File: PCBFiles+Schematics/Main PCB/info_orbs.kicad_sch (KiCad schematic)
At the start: 11 parts, among them SW1 SW_Push, SW2 SW_Push, SW3 SW_Push

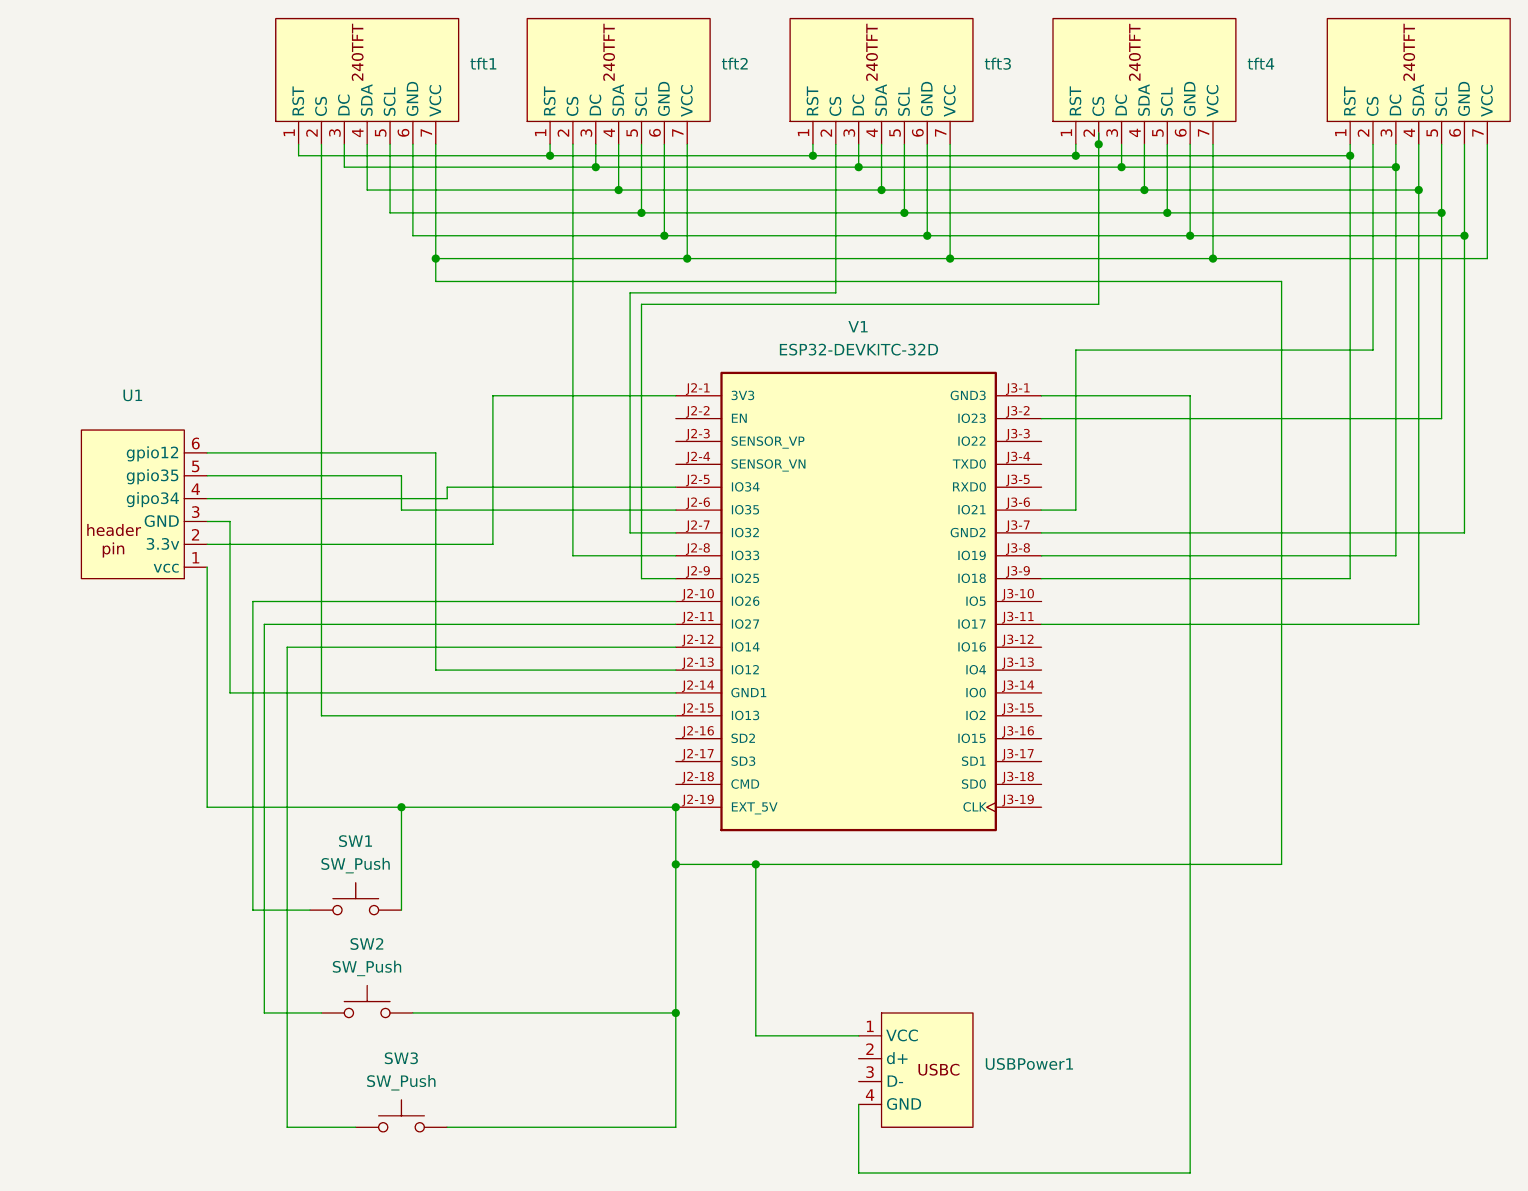
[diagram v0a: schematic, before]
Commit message: Updated New PCB Files
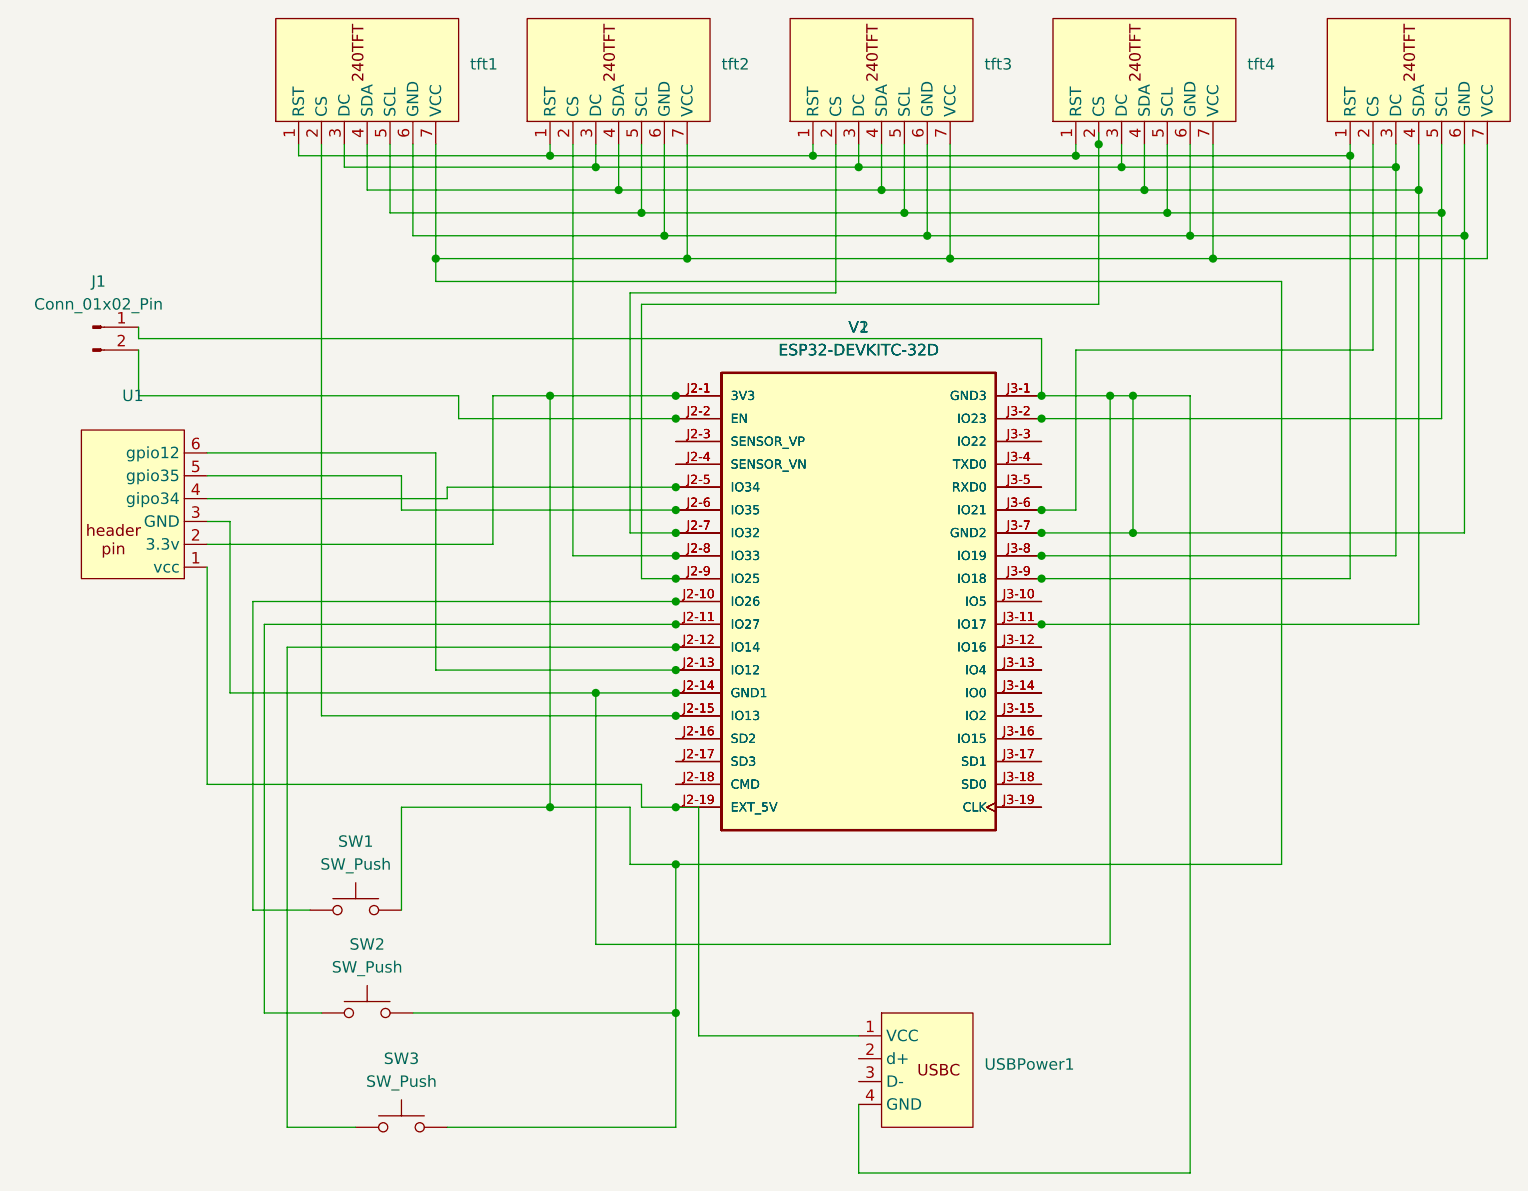
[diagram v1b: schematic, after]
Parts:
- added J1: Conn_01x02_Pin, Connector_PinHeader_2.54mm:PinHeader_1x02_P2.54mm_Vertical, symbol Connector:Conn_01x02_Pin
- added V2: ESP32-DEVKITC-32D, A Local Libs:38 Pin Board thin, symbol ESP32-DEVKITC-32D:ESP32-DEVKITC-32D
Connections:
- net at V1.J3-9 (IO18), tft1.1 (RST), tft2.1 (RST)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: now also V2.J3-9 (IO18)
- net at V1.J3-6 (IO21), tft5.2 (CS): now also V2.J3-6 (IO21)
- net at V1.J3-8 (IO19), tft1.3 (DC), tft2.3 (DC)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: now also V2.J3-8 (IO19)
- net at V1.J3-11 (IO17), tft1.4 (SDA), tft2.4 (SDA)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: now also V2.J3-11 (IO17)
- net at V1.J3-2 (IO23), tft1.5 (SCL), tft2.5 (SCL)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: now also V2.J3-2 (IO23)
- net at V1.J3-7 (GND2), tft1.6 (GND), tft2.6 (GND)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: now also U1.3 (GND), USBPower1.4 (GND), V1.J2-14 (GND1), V1.J3-1 (GND3), J1.1 (Pin_1), V2.J2-14 (GND1), V2.J3-1 (GND3), V2.J3-7 (GND2)
- net at SW1.2, SW2.2, SW3.2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: now also U1.2 (3.3v), V1.J2-1 (3V3), V2.J2-1 (3V3); no longer U1.1 (vcc), USBPower1.1 (VCC), V1.J2-19 (EXT_5V)
- net at V1.J2-7 (IO32), tft3.2 (CS): now also V2.J2-7 (IO32)
- net at U1.4 (gipo34), V1.J2-5 (IO34): now also V2.J2-5 (IO34)
- net at U1.5 (gpio35), V1.J2-6 (IO35): now also V2.J2-6 (IO35)
- net at U1.6 (gpio12), V1.J2-13 (IO12): now also V2.J2-13 (IO12)
- net at V1.J2-9 (IO25), tft4.2 (CS): now also V2.J2-9 (IO25)
- net at SW1.1, V1.J2-10 (IO26): now also V2.J2-10 (IO26)
- net at SW2.1, V1.J2-11 (IO27): now also V2.J2-11 (IO27)
- net at SW3.1, V1.J2-12 (IO14): now also V2.J2-12 (IO14)
- net at V1.J2-15 (IO13), tft1.2 (CS): now also V2.J2-15 (IO13)
- net at V1.J2-16 (SD2): now also V2.J2-16 (SD2)
- net at V1.J2-17 (SD3): now also V2.J2-17 (SD3)
- net at V1.J2-18 (CMD): now also V2.J2-18 (CMD)
- net at V1.J2-2 (EN): now also J1.2 (Pin_2), V2.J2-2 (EN)
- net at V1.J2-3 (SENSOR_VP): now also V2.J2-3 (SENSOR_VP)
- net at V1.J2-4 (SENSOR_VN): now also V2.J2-4 (SENSOR_VN)
- net at V1.J2-8 (IO33), tft2.2 (CS): now also V2.J2-8 (IO33)
- net at V1.J3-10 (IO5): now also V2.J3-10 (IO5)
- net at V1.J3-12 (IO16): now also V2.J3-12 (IO16)
- net at V1.J3-13 (IO4): now also V2.J3-13 (IO4)
- net at V1.J3-14 (IO0): now also V2.J3-14 (IO0)
- net at V1.J3-15 (IO2): now also V2.J3-15 (IO2)
- net at V1.J3-16 (IO15): now also V2.J3-16 (IO15)
- net at V1.J3-17 (SD1): now also V2.J3-17 (SD1)
- net at V1.J3-18 (SD0): now also V2.J3-18 (SD0)
- net at V1.J3-19 (CLK): now also V2.J3-19 (CLK)
- net at V1.J3-3 (IO22): now also V2.J3-3 (IO22)
- net at V1.J3-4 (TXD0): now also V2.J3-4 (TXD0)
- net at V1.J3-5 (RXD0): now also V2.J3-5 (RXD0)
- new net: U1.1 (vcc), USBPower1.1 (VCC), V1.J2-19 (EXT_5V), V2.J2-19 (EXT_5V)
